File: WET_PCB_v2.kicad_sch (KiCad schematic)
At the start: 24 parts, among them J10 Conn_01x09_Pin, J11 Conn_01x09_Pin, J2 Conn_01x09_Pin, J3 Conn_01x09_Pin, J4 XT60, J5 Barrel jack, J6 Pluggable Terminal Block, J7 Pluggable Terminal Block, J8 Jumper, U3 Opamp_Quad

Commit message: SCH Save: 1 files changed WET_PCB_v2.kicad_sch 0/0/1
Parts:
- J7: footprint (none) -> Connector_Phoenix_GMSTB:PhoenixContact_GMSTBA_2,5_2-G-7,62_1x02_P7.62mm_Horizontal
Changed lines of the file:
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@@
 			)
 		)
-		(property "Footprint" ""
+		(property "Footprint" "Connector_Phoenix_GMSTB:PhoenixContact_GMSTBA_2,5_2-G-7,62_1x02_P7.62mm_Horizontal"
 			(at 245.11 26.67 0)
 			(hide yes)

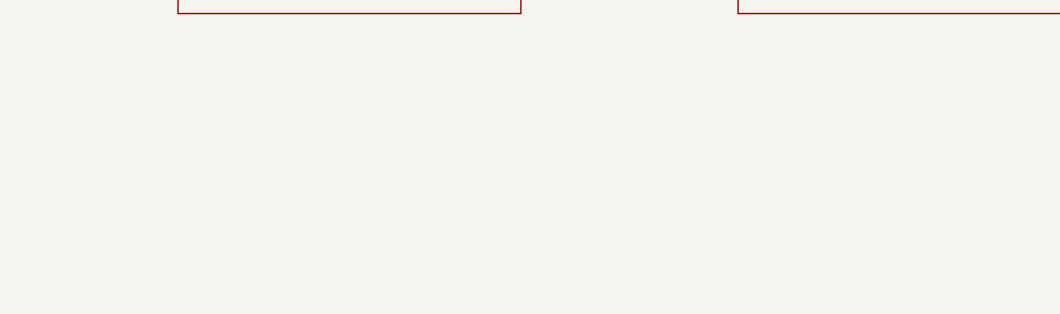
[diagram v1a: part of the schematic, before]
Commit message: SCH Save: 1 files changed WET_PCB_v2.kicad_sch 10/0/0
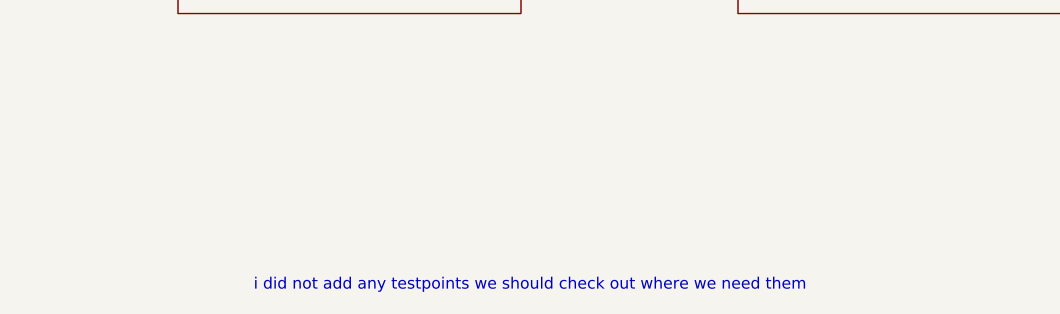
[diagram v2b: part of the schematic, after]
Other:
- note added: "i did not add any testpoints we should check out where we need them"
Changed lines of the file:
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@@
+		)
+	)
+	(text "i did not add any testpoints we should check out where we need them"
+		(exclude_from_sim no)
+		(at 178.816 122.936 0)
+		(effects
+			(font
+				(size 1.27 1.27)
+			)
 		)
 	)

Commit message: most footprints added (some random)
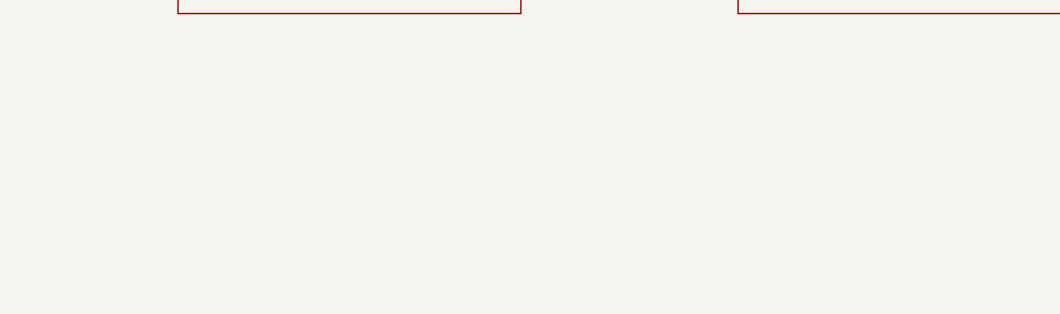
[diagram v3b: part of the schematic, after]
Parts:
- J7: footprint Connector_Phoenix_GMSTB:PhoenixContact_GMSTBA_2,5_2-G-7,62_1x02_P7.62mm_Horizontal -> (none)
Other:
- note removed: "i did not add any testpoints we should check out where we need them"
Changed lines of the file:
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@@
-		)
-	)
-	(text "i did not add any testpoints we should check out where we need them"
-		(exclude_from_sim no)
-		(at 178.816 122.936 0)
-		(effects
-			(font
-				(size 1.27 1.27)
-			)
 		)
 	)
@@
 			)
 		)
-		(property "Footprint" "Connector_Phoenix_GMSTB:PhoenixContact_GMSTBA_2,5_2-G-7,62_1x02_P7.62mm_Horizontal"
+		(property "Footprint" ""
 			(at 245.11 26.67 0)
 			(hide yes)
